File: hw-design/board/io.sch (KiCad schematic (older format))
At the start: 29 parts, among them P3 FOOT, P4 FOOT, P5 FOOT, P6 FOOT, U5 PCA9685

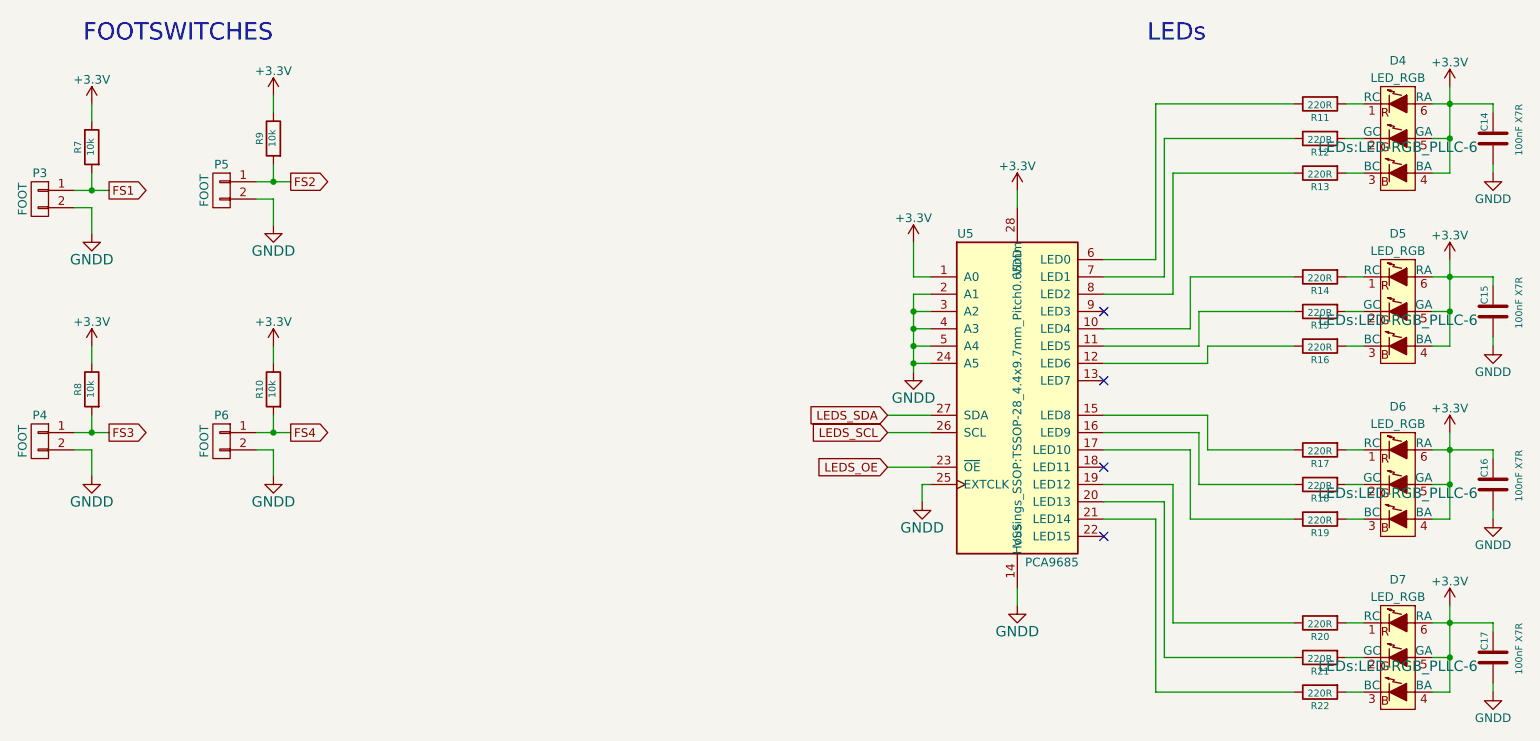
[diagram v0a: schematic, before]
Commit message: connecting foot leds directly to cpu
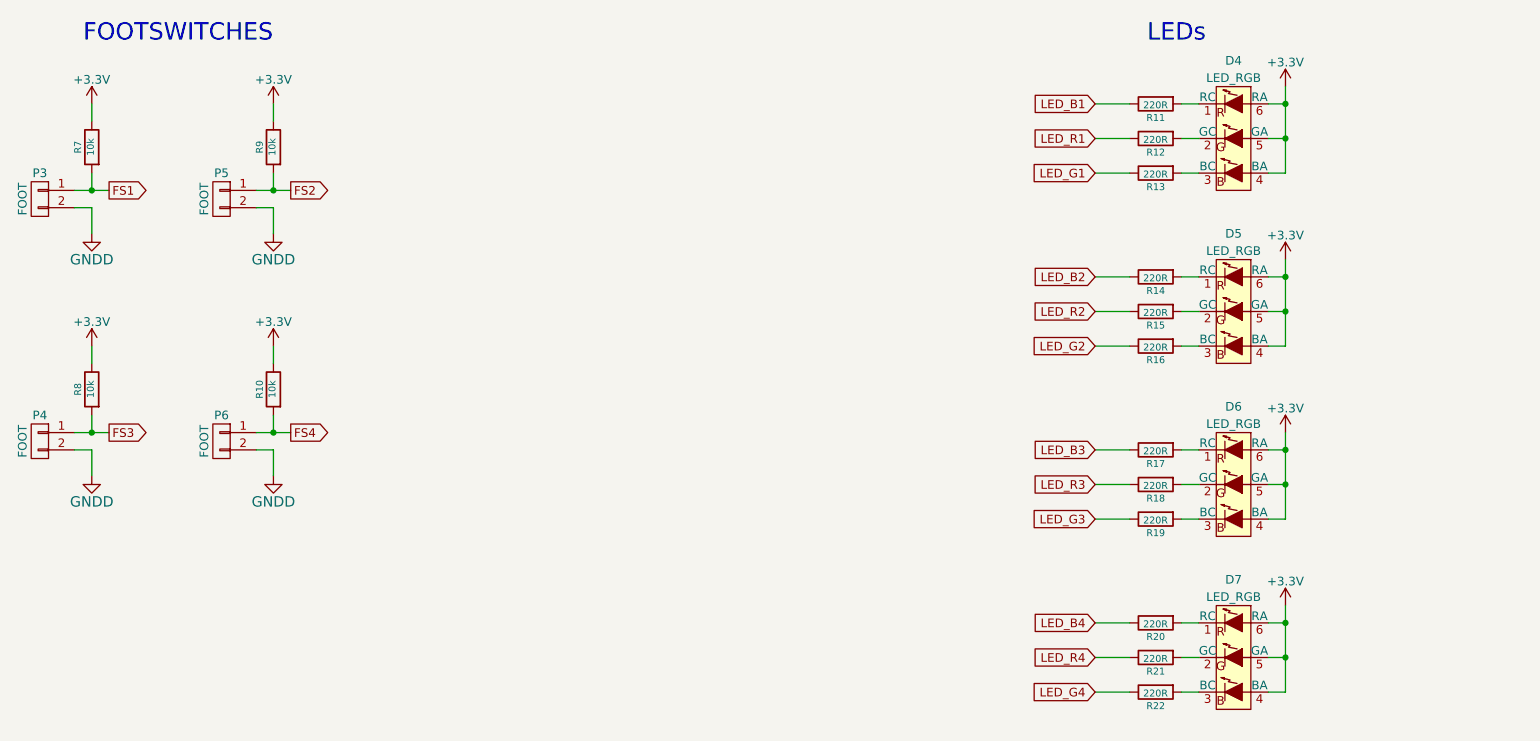
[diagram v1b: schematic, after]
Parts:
- removed C14, C15, C16, C17: 100nF X7R, Capacitors_SMD:C_0603, symbol C
- removed U5: PCA9685, Housings_SSOP:TSSOP-28_4.4x9.7mm_Pitch0.65mm, symbol PCA9685
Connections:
- net LED_B1: now reaches R11.1
- net LED_R1: now reaches R12.1
- net LED_G1: now reaches R13.1
- net LED_B2: now reaches R14.1
- net LED_R2: now reaches R15.1
- net LED_G2: now reaches R16.1
- net LED_B3: now reaches R17.1
- net LED_R3: now reaches R18.1
- net LED_G3: now reaches R19.1
- net LED_B4: now reaches R20.1
- net LED_R4: now reaches R21.1
- net LED_G4: now reaches R22.1
- no-connect marks 4 -> 0
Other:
- moved on the sheet: D4, D5, D6, D7, P5, R11, R12, R13, R14, R15, R16, R17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
